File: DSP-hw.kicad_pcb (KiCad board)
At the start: 4 copper layers, 184 x 65.6 mm, 107 parts, among them J1 NC3MAH, J10 AudioJack3, J11 AudioJack3, J2 NC3MAH, J3 NC3MAH, J4 NC3MAH, J5 XLR3_AudioJack3_Combo_Ground, J6 XLR3_AudioJack3_Combo_Ground, J7 USB_C_Receptacle_USB2.0_16P, J8 Conn_01x04_Pin, J9 Conn_01x06_Pin, Q1 BC327, Q2 AO3400A, SW1 SW_Push, SW2 SW_Push, SW6 SW_SPST, SW7 SW_SPST, SW8 SW_Push, U1 ADAU1701, U2 CAT24C256, U3 AMS1117-3.3, U4 STM32F411RETx, U5 TME-0505S, U6 ADUM3160, Y1 12.228M

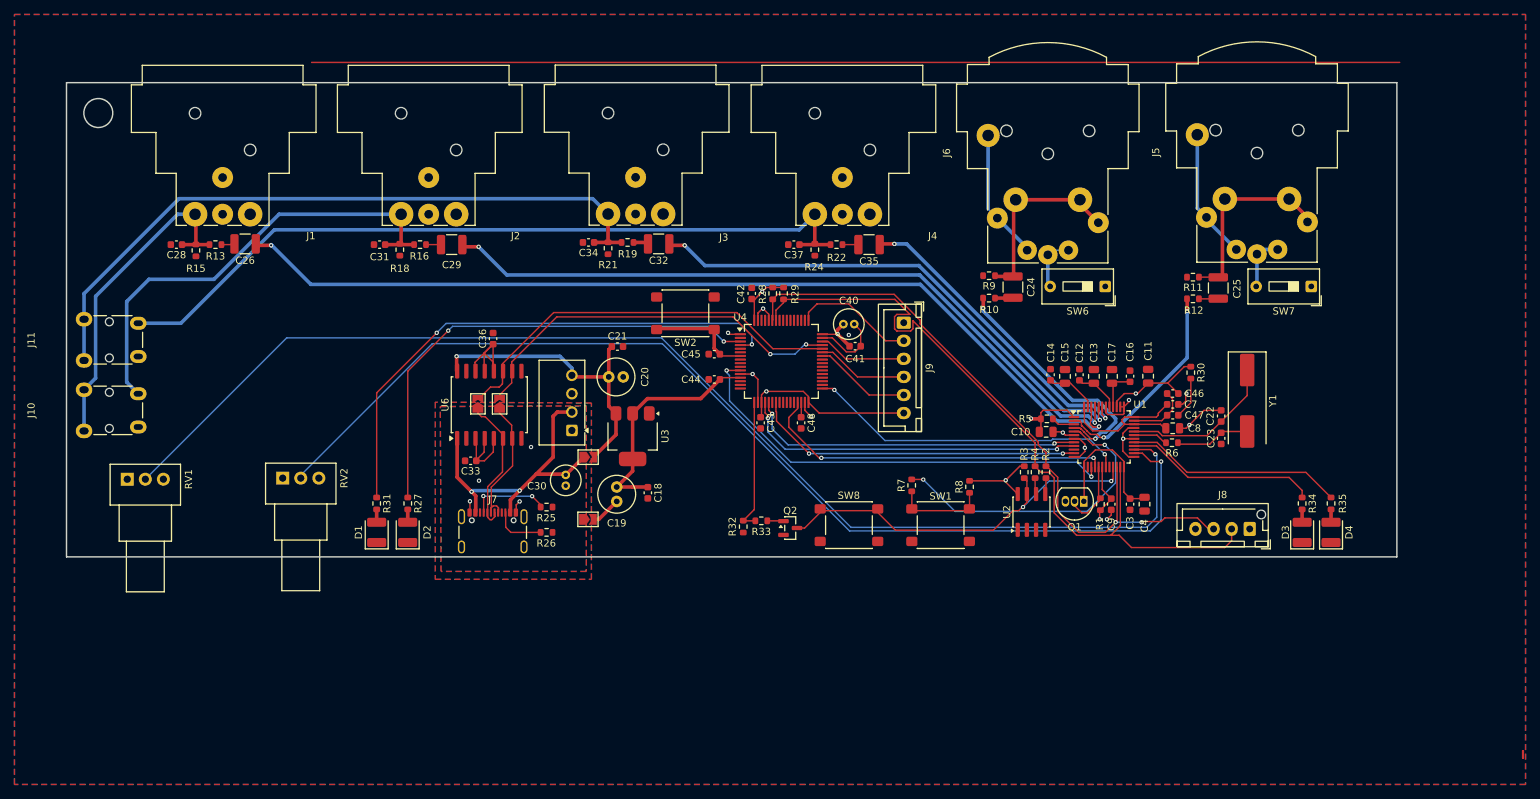
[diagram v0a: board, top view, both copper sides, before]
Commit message: passato tutto a due layer
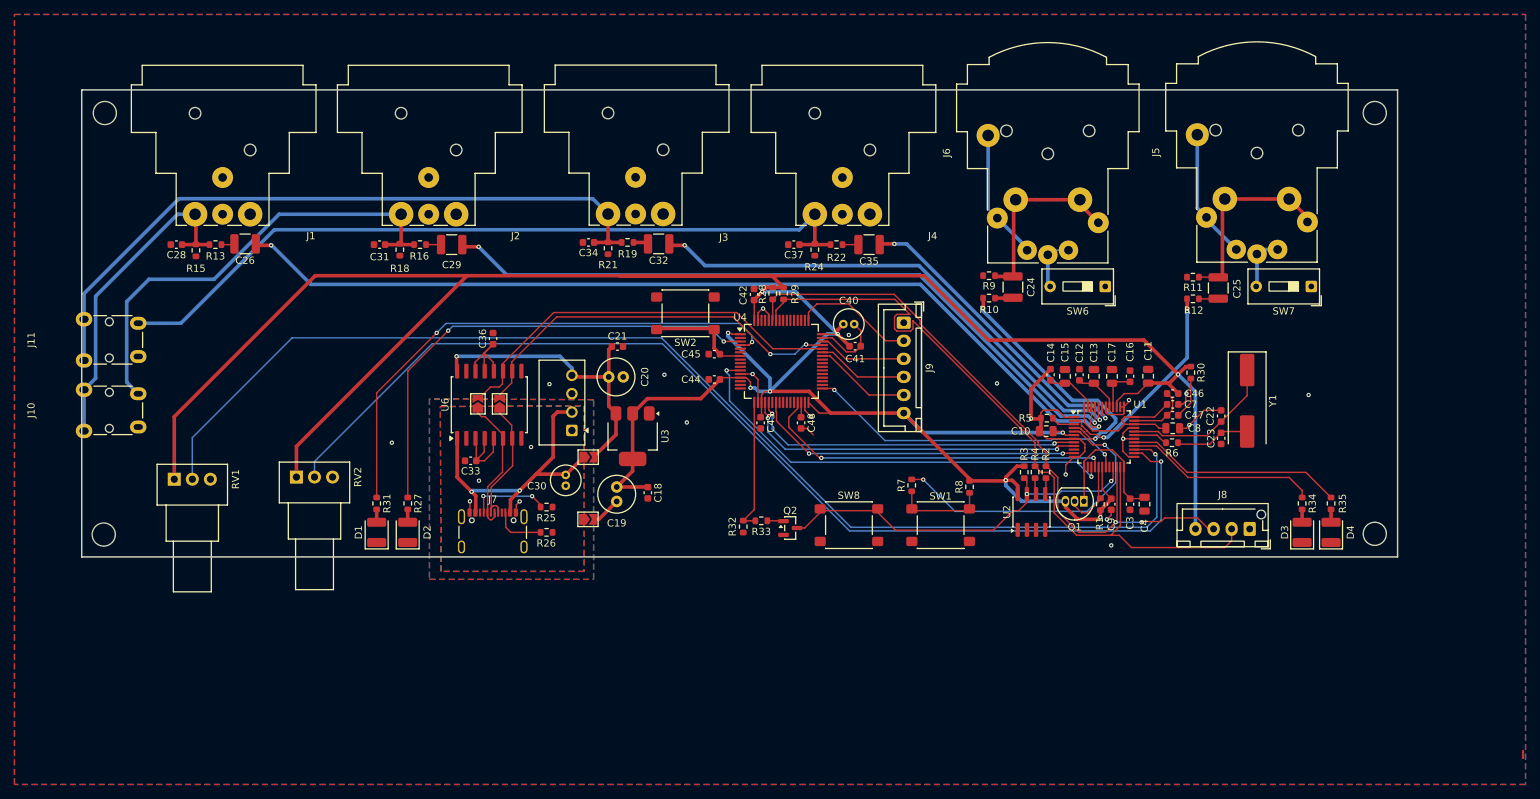
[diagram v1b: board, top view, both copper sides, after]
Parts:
- moved RV1 6.50 mm to (73.0, 83.7)
- moved RV2 1.91 mm to (89.9, 83.3)
- moved C42 0.36 mm to (153.2, 58.1)
- moved C10 0.10 mm to (193.6, 77.0)
- moved R5 0.10 mm to (193.7, 75.2)
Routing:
- net +3V3: track 111.1 -> 453.6 mm, vias 8 -> 9
- net GND: track 64.8 -> 83.0 mm, vias 11 -> 18
- net Net-(U6-PIN): track 15.8 -> 12.1 mm
- net /MP8: track 171.4 -> 168.3 mm
- net /WP: track 54.7 -> 53.5 mm
- net /MP9: track 150.6 -> 149.7 mm
- removed copper zone on In1.Cu, net +3V3
- removed copper zone on In2.Cu, net +3V3
- removed copper zone on In1.Cu, net GND
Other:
- board size 184 x 65.6 mm -> 182 x 64.6 mm
- copper layers 4 -> 2
